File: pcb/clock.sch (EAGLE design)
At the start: 54 parts, among them K1 JS-M1-9V-4, K2 JS-M1-9V-4, Q1 BC447, Q2 BC447, Q3 BC447, Q4 BC447, Q5 BC447, Q6 BC447, Q8 CSM-7X-DU, Q9 MC-306, U1 ATMEGA328P-AU, U2 PCF8563T/F4

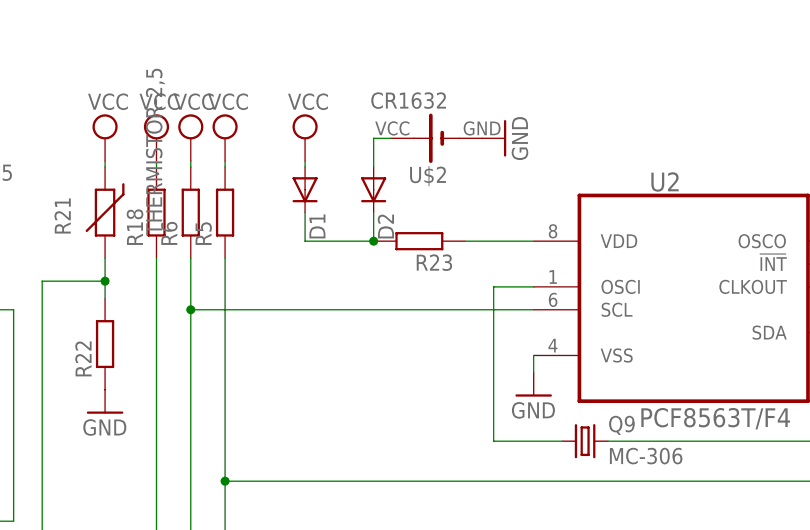
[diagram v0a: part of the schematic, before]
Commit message: temp stable version
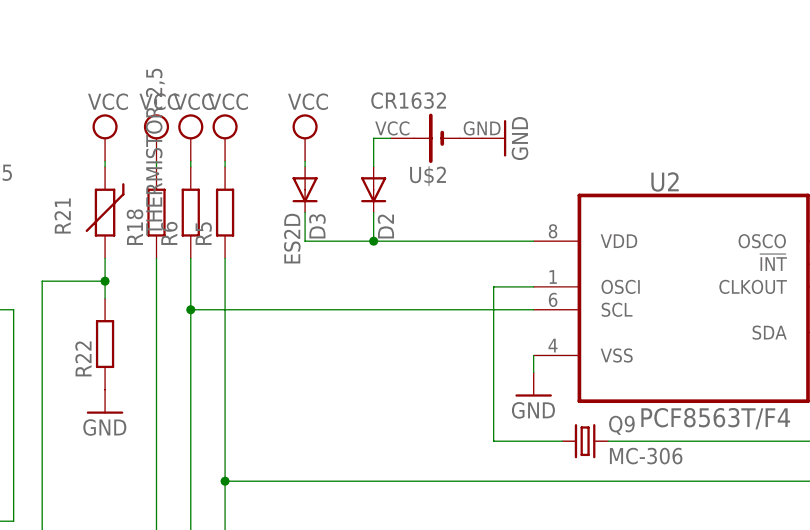
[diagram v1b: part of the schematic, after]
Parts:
- removed D1: (no value), diode:DIODE-SOD80C
- removed R23: (no value), rcl:R-EU_R1206
- added D3: ES2D, diode:ES2D
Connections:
- removed net N$68: R23.1, U2.VDD
- net N$67: now also D3.C, U2.VDD; no longer D1.C, R23.2
- net VCC: now also D3.A; no longer D1.A
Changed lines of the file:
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@@
 <part name="GND22" library="supply1" deviceset="GND" device=""/>
 <part name="C7" library="rcl" deviceset="C-EU" device="025-040X050"/>
-<part name="D1" library="diode" deviceset="DIODE-" device="SOD80C"/>
-<part name="R23" library="rcl" deviceset="R-EU_" device="R1206"/>
 <part name="C6" library="rcl" deviceset="C-EU" device="C0805K"/>
 <part name="C3" library="rcl" deviceset="C-EU" device="C0805K"/>
+<part name="D3" library="diode" deviceset="ES2D" device=""/>
 </parts>
 <sheets>
@@
 <instance part="GND22" gate="1" x="34.925" y="63.5" rot="R270"/>
 <instance part="C7" gate="G$1" x="40.64" y="73.66"/>
-<instance part="D1" gate="G$1" x="118.745" y="115.57" rot="R270"/>
-<instance part="R23" gate="G$1" x="131.445" y="109.855" rot="R180"/>
 <instance part="C6" gate="G$1" x="38.1" y="43.18" rot="R90"/>
 <instance part="C3" gate="G$1" x="38.1" y="38.1" rot="R90"/>
+<instance part="D3" gate="G$1" x="118.745" y="115.57" rot="R270"/>
 </instances>
 <busses>
@@
 <segment>
 <pinref part="SUPPLY6" gate="G$1" pin="VCC"/>
-<pinref part="D1" gate="G$1" pin="A"/>
 <wire x1="118.745" y1="118.11" x2="118.745" y2="118.745" width="0.1524" layer="91"/>
+<pinref part="D3" gate="G$1" pin="A"/>
 </segment>
 </net>
@@
 <wire x1="126.365" y1="109.855" x2="126.365" y2="113.03" width="0.1524" layer="91"/>
 <wire x1="118.745" y1="109.855" x2="126.365" y2="109.855" width="0.1524" layer="91"/>
-<pinref part="D1" gate="G$1" pin="C"/>
 <wire x1="118.745" y1="109.855" x2="118.745" y2="113.03" width="0.1524" layer="91"/>
-<pinref part="R23" gate="G$1" pin="2"/>
+<pinref part="D3" gate="G$1" pin="C"/>
+<pinref part="U2" gate="A" pin="VDD"/>
+<wire x1="126.365" y1="109.855" x2="144.145" y2="109.855" width="0.1524" layer="91"/>
 <junction x="126.365" y="109.855"/>
 </segment>
 </net>
-<net name="N$68" class="0">
-<segment>
-<pinref part="U2" gate="A" pin="VDD"/>
-<pinref part="R23" gate="G$1" pin="1"/>
-<wire x1="136.525" y1="109.855" x2="144.145" y2="109.855" width="0.1524" layer="91"/>
-</segment>
-</net>
